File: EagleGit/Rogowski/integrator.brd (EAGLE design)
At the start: 60.9 x 84.8 mm, 25 parts, among them IC1 TL061P, IC2 TL061P

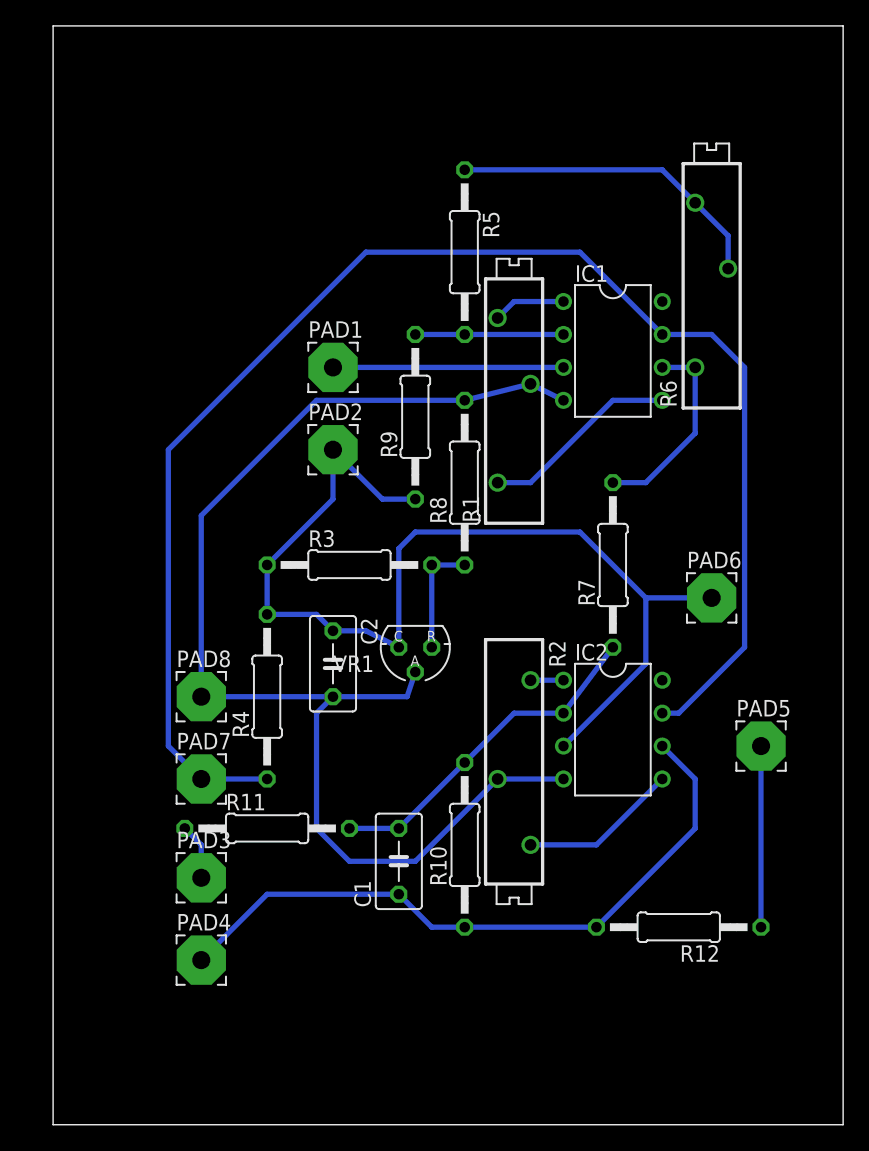
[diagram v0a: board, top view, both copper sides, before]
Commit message: DPS pro akvarko
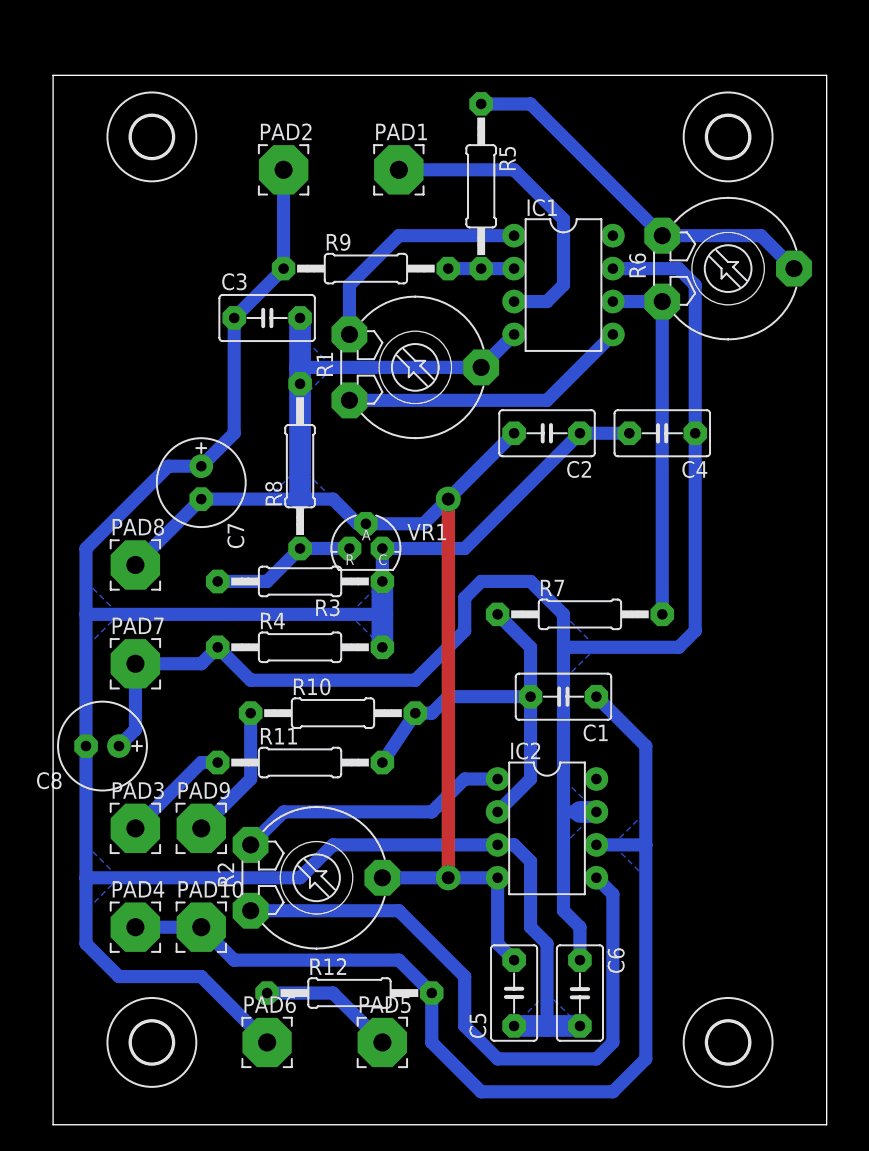
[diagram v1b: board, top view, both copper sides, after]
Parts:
- added C3, C4, C5, C6: (no value), rcl:C050-035X075
- added C7, C8: (no value), rcl:E2,5-7
- added PAD10, PAD9: (no value), wirepad:3,81/1,4
- added U$1, U$2, U$3, U$4: (no value), holes:3,2
- R1, R2, R6: device rcl:RTRIMT18 -> pot:LI10
- moved PAD6 48.5 mm to (16.5, 6.35)
- moved PAD5 37.1 mm to (25.4, 6.35)
- moved R12 25.9 mm to (22.9, 10.2), turned to 0 degrees
- moved C2 24.3 mm to (38.1, 53.3), turned to 180 degrees
- moved PAD2 21.9 mm to (17.8, 73.7)
- moved C1 18.0 mm to (39.4, 33.0), turned to 180 degrees
- moved R2 17.0 mm to (20.3, 19.1)
- moved PAD1 16.1 mm to (26.7, 73.7)
- moved R10 14.4 mm to (21.6, 31.8), turned to 0 degrees
- moved R8 12.8 mm to (19.1, 50.8)
- moved R9 12.0 mm to (24.1, 66.0), turned to 0 degrees
- moved PAD8 11.4 mm to (6.35, 43.2)
- moved PAD7 10.2 mm to (6.35, 35.6)
- moved IC2 9.16 mm to (38.1, 22.9)
- moved VR1 8.52 mm to (24.1, 44.5), turned to 0 degrees
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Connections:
- removed net N$9: C1.1, IC2.6, PAD4.1, R10.1, R12.2
- new net N$11: PAD9.1, R10.1
- new net OUT: C1.1, IC2.6, PAD10.1, PAD4.1, R12.2
- net GND: now also C3.2, C5.2, C7.-, R1.S, R2.S; no longer R1.2, R2.2
- net GND2: now also C3.1, C4.2, C5.1, C6.2, C7.+, C8.-
- net N$1: now also R1.E; no longer R1.1
- net N$2: now also R1.A; no longer R1.3
- net N$3: now also R2.E; no longer R2.3
- net N$4: now also R2.A; no longer R2.1
- net N$6: now also R6.A, R6.S; no longer R6.2, R6.3
- net N$7: now also R6.E; no longer R6.1
- net VDD: now also C4.1, C6.1, C8.+
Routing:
- net GND2: track 82.2 -> 192.0 mm
- net OUT: track 0.00 -> 81.2 mm
- net N$9: track 51.8 -> 0.00 mm
- net N$3: track 12.3 -> 48.7 mm
- net N$4: track 2.54 -> 21.2 mm
- net GND: track 97.3 -> 111.5 mm, vias 0 -> 2
- net N$2: track 5.61 -> 18.1 mm
- net N$7: track 15.5 -> 27.9 mm
- net N$11: track 0.00 -> 10.5 mm
- net N$1: track 15.3 -> 22.4 mm
- net N$5: track 11.4 -> 5.08 mm
- net N$14: track 17.8 -> 23.7 mm
- net VDD: track 116.0 -> 121.1 mm
- net N$8: track 26.5 -> 31.3 mm
- net N$6: track 25.0 -> 29.4 mm
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- added copper zone on layer 16, net GND
- added copper zone on layer 16, net GND2
- added copper zone on layer 16, net OUT
- added copper zone on layer 16, net VDD
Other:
- board size 60.9 x 84.8 mm -> 59.7 x 81 mm
